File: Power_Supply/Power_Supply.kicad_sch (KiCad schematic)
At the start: 69 parts, among them J1 Conn_01x03_Pin, J2 Conn_01x03_Pin, J3 Conn_01x03_Pin, J4 5745782-6, J7 1287, J8 1287, J9 1287, K2 G5LE-1, Q1 2N7000, U3 Fuse, 1A, U4 Fuse, 5A, U5 traco_TSR_0.5-2433, U6 LM75C

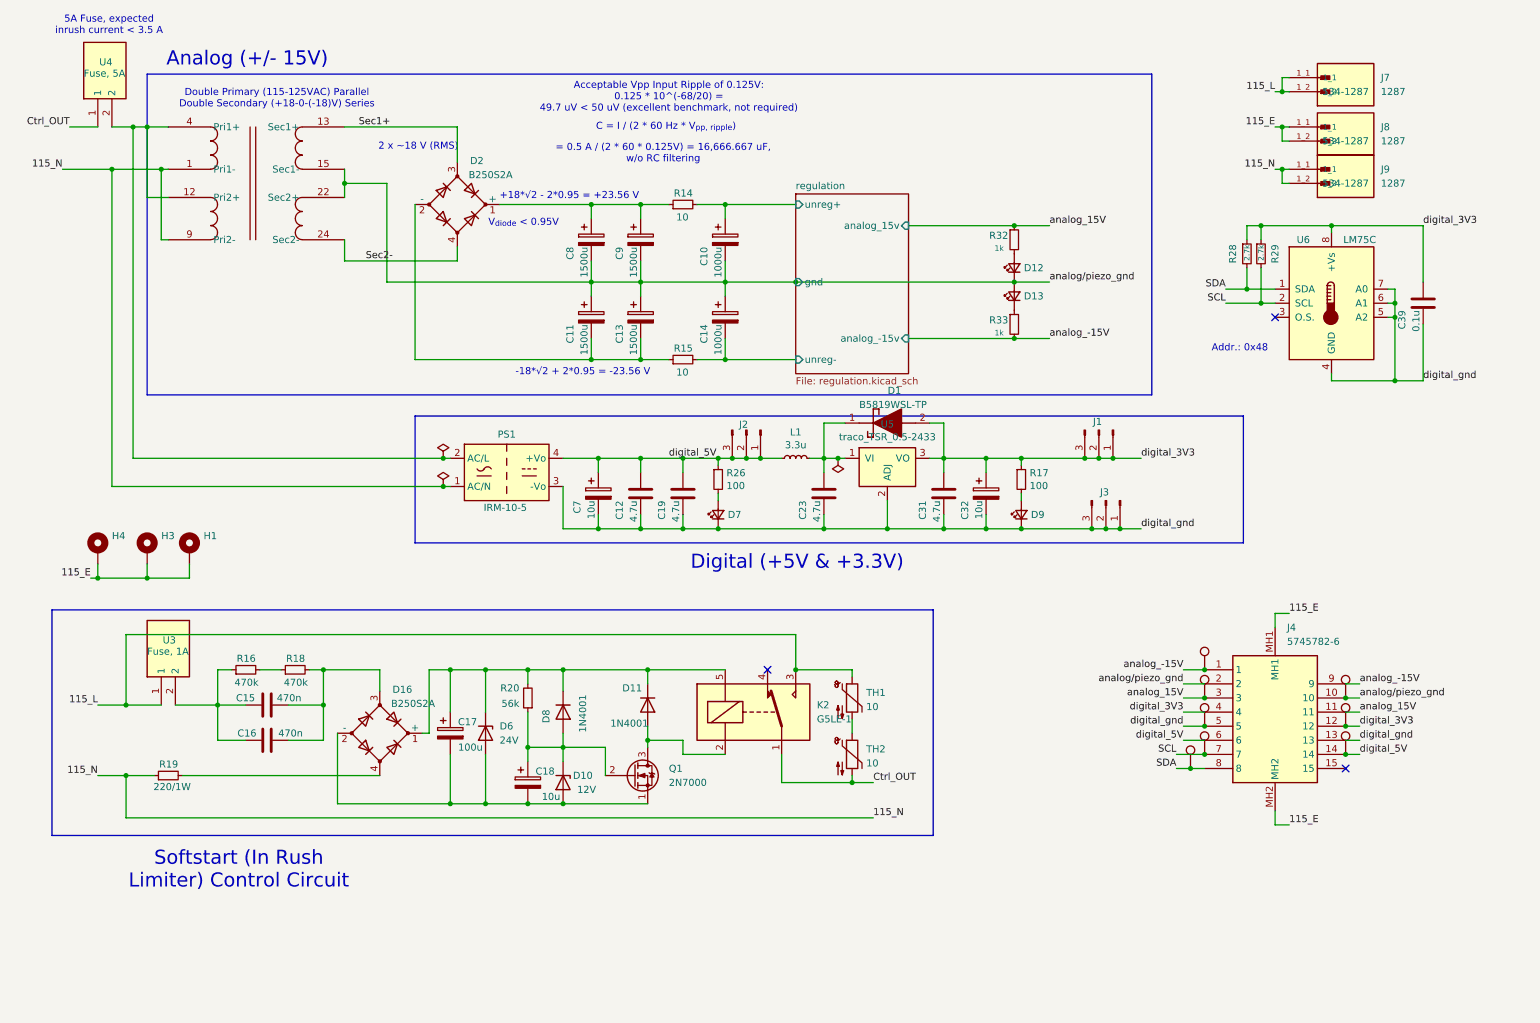
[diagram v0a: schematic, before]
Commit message: Analog Circuit V1.0
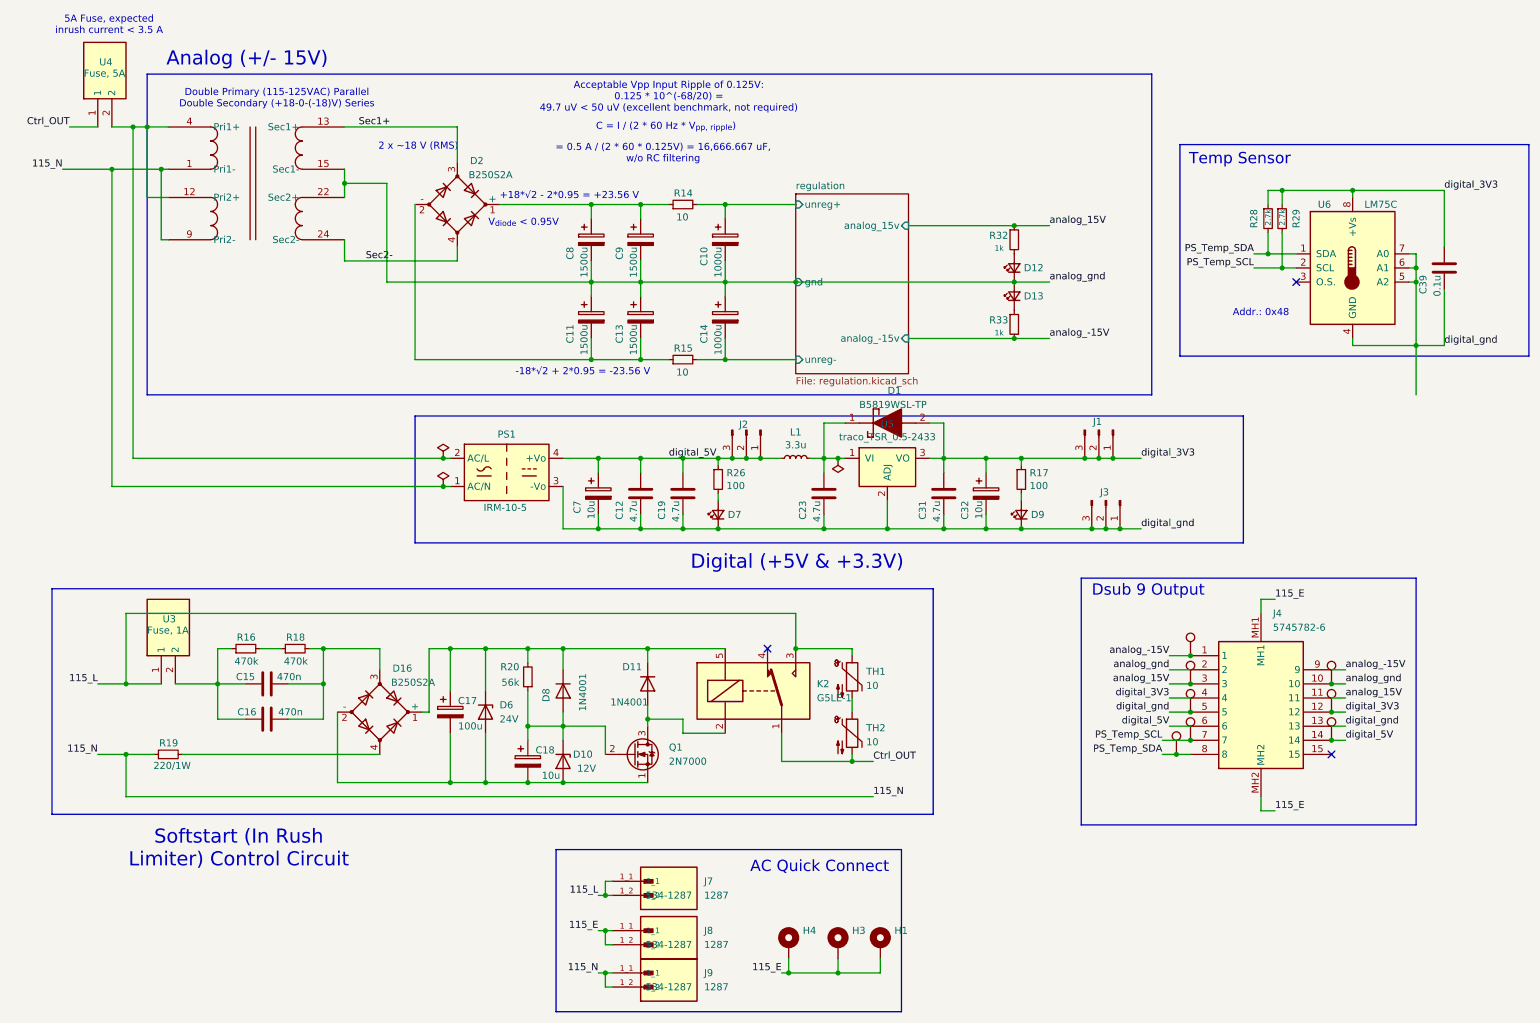
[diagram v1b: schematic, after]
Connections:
- net SCL renamed PS_Temp_SCL
- net SDA renamed PS_Temp_SDA
- net analog/piezo_gnd renamed analog_gnd
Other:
- note added: "AC Quick Connect"
- note added: "Dsub 9 Output"
- note added: "Temp Sensor"
- moved on the sheet: C15, C16, C17, C18, C39, D10, D11, D16, D6, D8, H1, H3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
